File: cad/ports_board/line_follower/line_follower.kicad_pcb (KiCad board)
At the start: 2 copper layers, 50 x 22 mm, 7 parts, among them J2 Conn_01x03, J5 Conn_01x03, J7 Conn_01x03, J8 Conn_01x03, J9 Conn_01x06_MountingPin

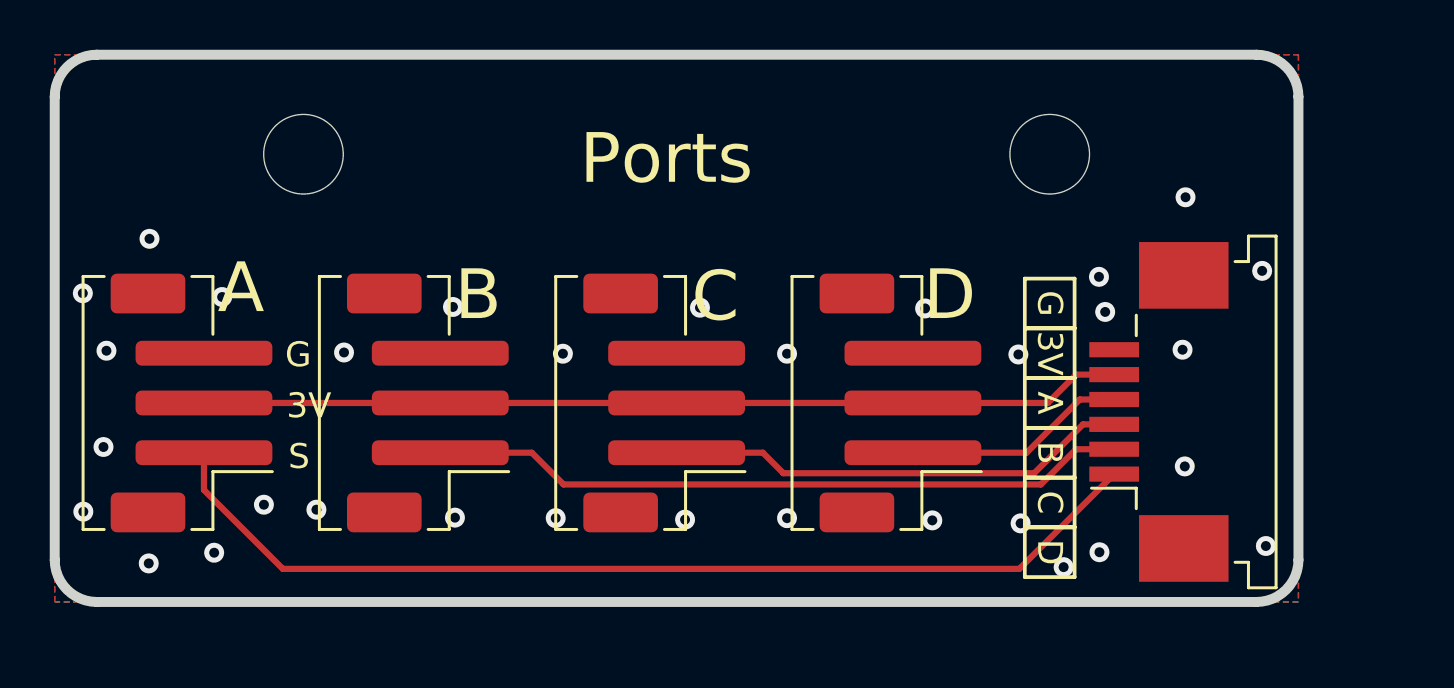
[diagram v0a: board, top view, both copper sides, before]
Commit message: Big Kahuna finished, winrar zippy files are funny
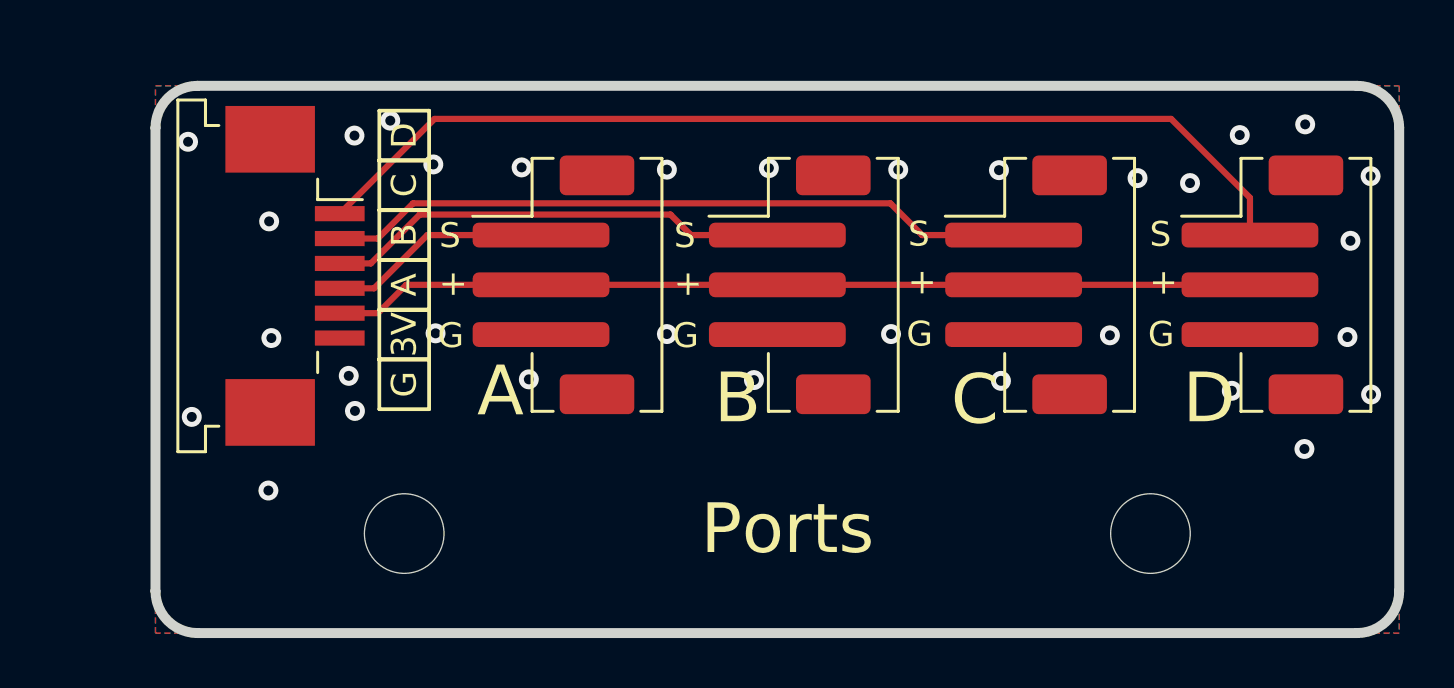
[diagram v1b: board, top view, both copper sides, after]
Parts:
- moved J2 43.3 mm to (188.6, 80.2), turned to -90 degrees
- moved H2 37.3 mm to (184.1, 90.2), turned to 180 degrees
- moved J9 35.2 mm to (149.7, 79.9), turned to -90 degrees
- moved H1 30.1 mm to (154.1, 90.2), turned to 180 degrees
- moved J5 24.5 mm to (179.1, 80.2), turned to -90 degrees
- moved J8 14.7 mm to (160.1, 80.2), turned to -90 degrees
- moved J7 6.93 mm to (169.6, 80.2), turned to -90 degrees
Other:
- board text added: "+"
